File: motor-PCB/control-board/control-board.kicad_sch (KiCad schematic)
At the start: 22 parts, among them J1 Power Input, J2 Motor, J3 Optocoupler, J4 Conn_01x04, J5 Connection with second PCB, U1 LM7812_TO220, U2 INA219BxDCN, U3 LM7805_TO220, U4 TMP117xxDRV

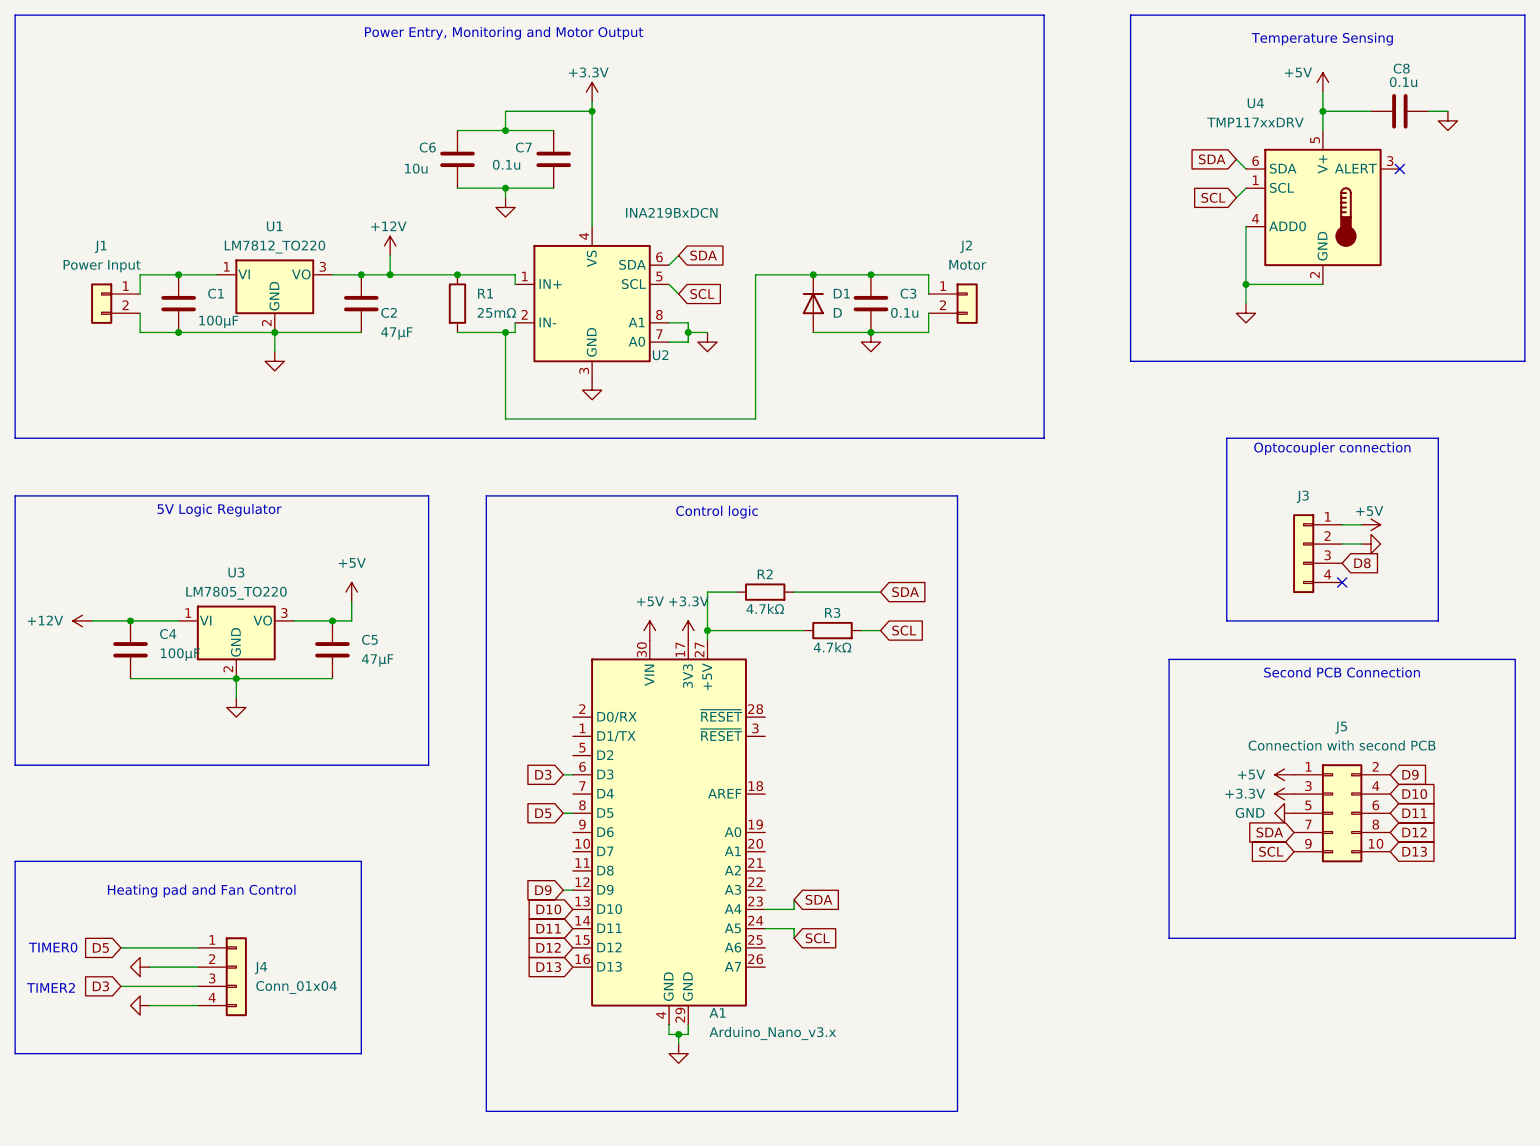
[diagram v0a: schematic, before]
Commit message: Final Control-Board
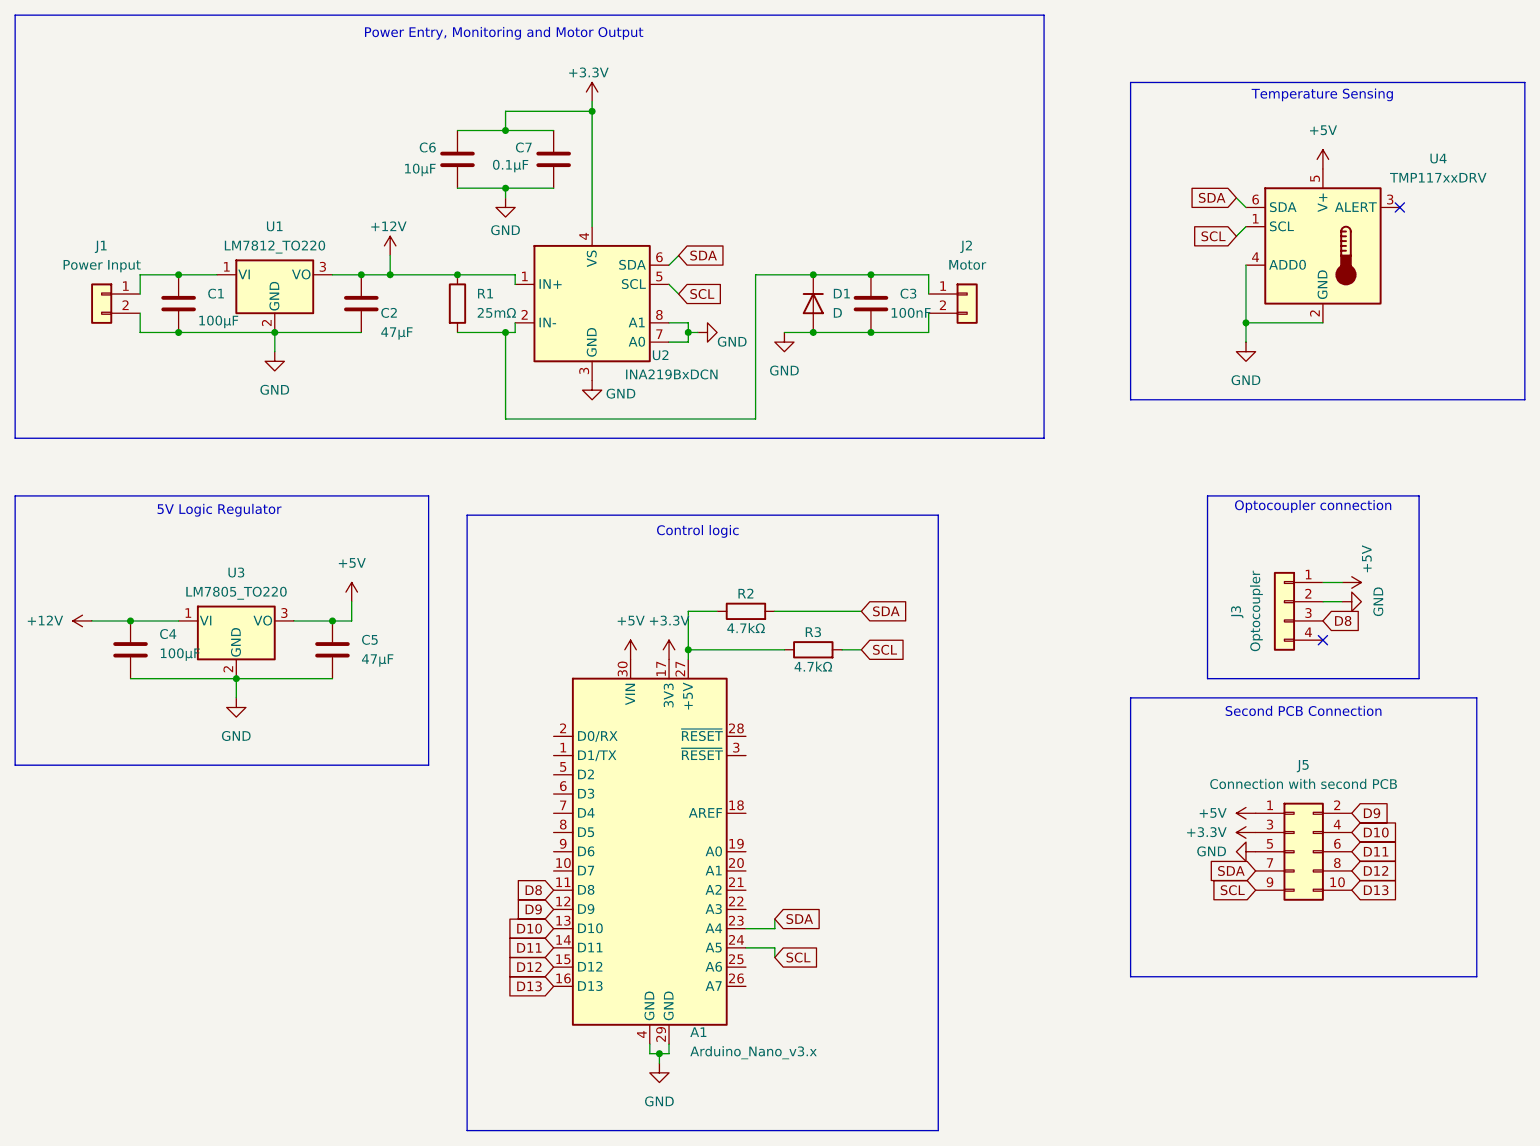
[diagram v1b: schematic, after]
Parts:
- removed C8: 0.1u, Capacitor_THT:C_Disc_D5.0mm_W2.5mm_P2.50mm, symbol Device:C
- removed J4: Conn_01x04, Custom:1x04_P2.54mm_Horizontal, symbol Connector_Generic:Conn_01x04
- C3: value 0.1u -> 100nF
- C6: value 10u -> 10µF
- C7: value 0.1u -> 0.1µF
- J1, J2: footprint Custom:1x02_P2.54mm_Horizontal -> TerminalBlock_CUI:TerminalBlock_CUI_TB007-508-02_1x02_P5.08mm_Horizontal
- R1: footprint Resistor_THT:R_Axial_DIN0414_L11.9mm_D4.5mm_P15.24mm_Horizontal -> Resistor_THT:R_Axial_DIN0414_L11.9mm_D4.5mm_P15.24mm_Horizonta
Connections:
- net D8: now also A1.11 (D8)
- net D3: no longer names the net of A1.6 (D3)
- net D5: no longer names the net of A1.8 (D5)
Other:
- note removed: "Heating pad and Fan Control"
- note removed: "TIMER0"
- note removed: "TIMER2"
- moved on the sheet: A1, J3, J5, R2, R3, U4
